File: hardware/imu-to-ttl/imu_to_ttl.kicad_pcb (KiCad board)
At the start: 2 copper layers, 41 x 30 mm, 58 parts, among them J1 BATT IN 2.54 2P, J2 SWD+UART+NRST, J3 J_NECK, J4 J_L, J5 J_R, Q1 AO4407C, U1 STM32G031F8P6, U2 LSM6DSV16XTR, U3 SN74LVC2G241DCUR, U4 HT7533-1

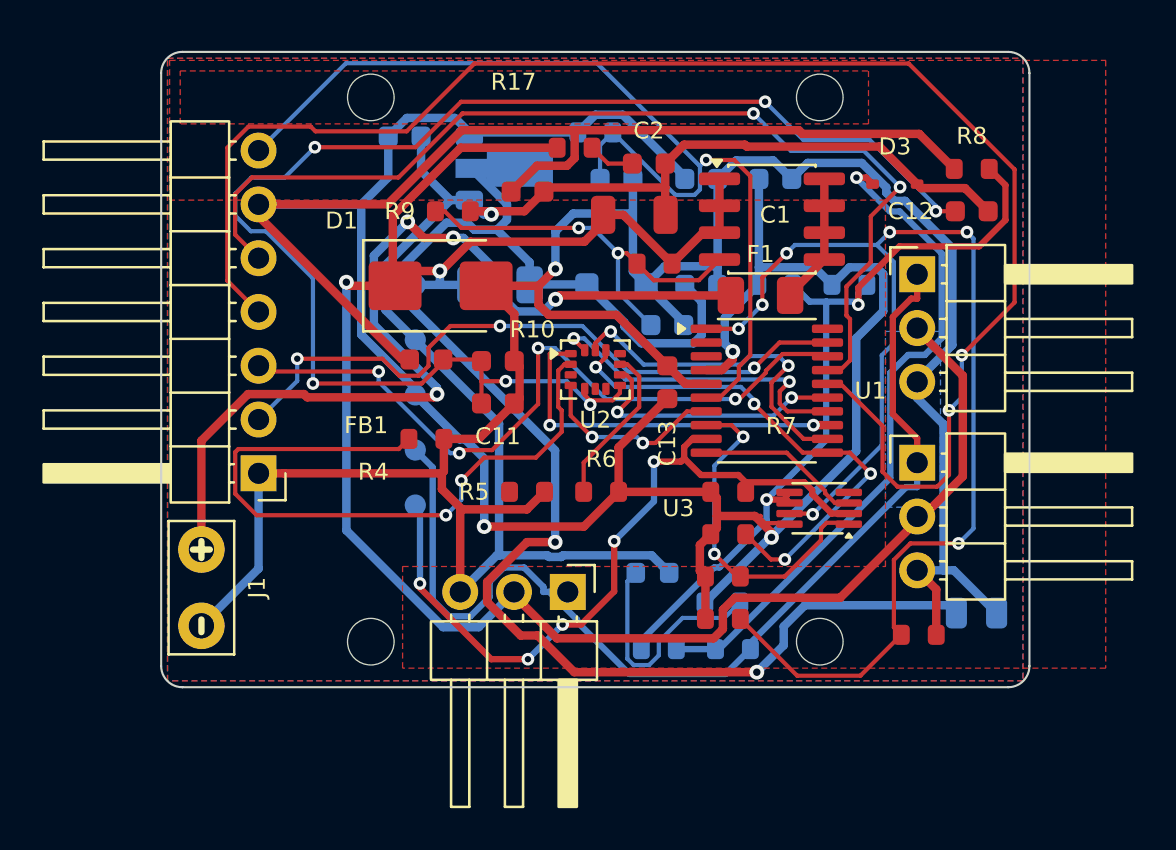
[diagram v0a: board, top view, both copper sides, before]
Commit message: sync: 2026-10-21 日常更新
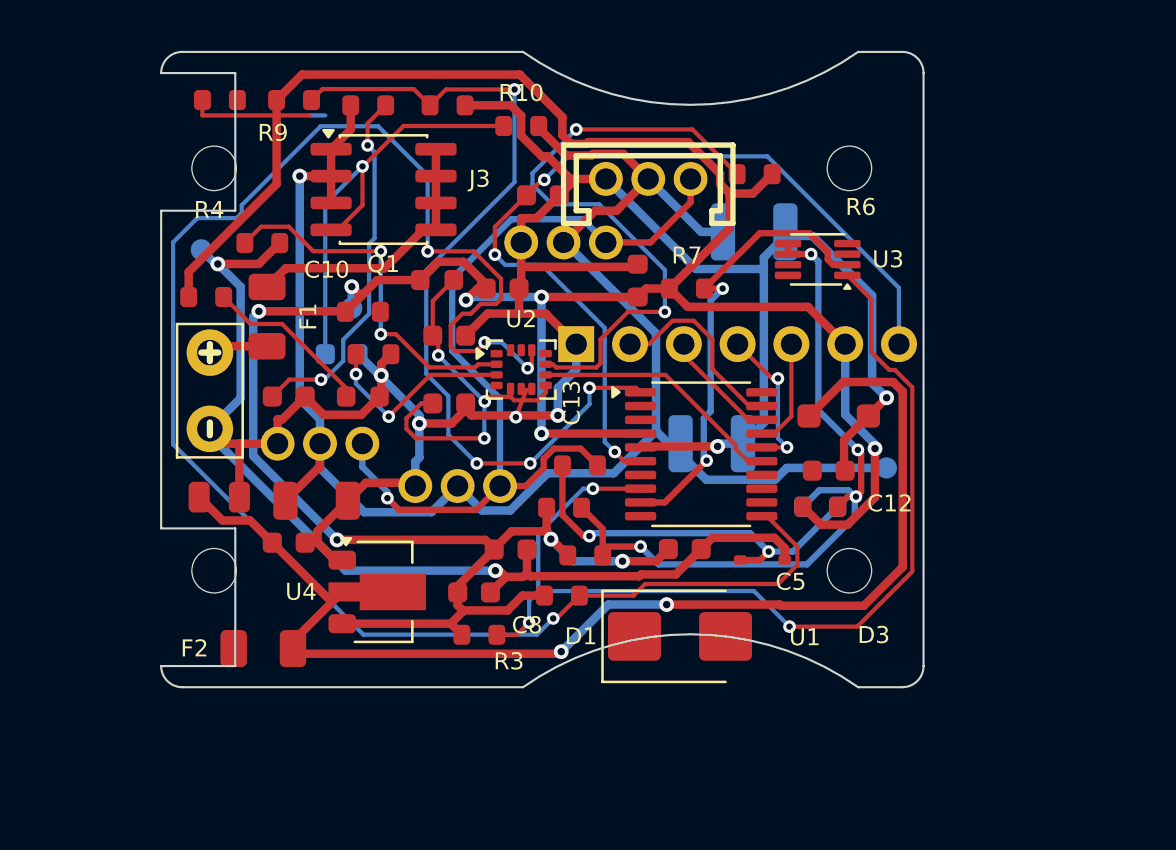
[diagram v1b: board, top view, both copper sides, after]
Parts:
- removed B1, B2, B3, B4: M2, MountingHole_2.2mm_M2
- removed TP4: BUS_DATA, TestPoint_Pad_D1.0mm
- removed TP5: BUS_TX, TestPoint_Pad_D1.0mm
- added C15: 22uF 16V X5R, C_1210_3225Metric, B.Cu at (26.0, 18.5)
- added C16: 22uF 16V X5R, C_1210_3225Metric, B.Cu at (28.0, 8.50)
- added J6: J_HEAD, CONN-TH_B3B-PH-K-S, B.Cu at (7.50, 18.5)
- added M1: M2, MountingHole_2.1mm_M2, F.Cu at (2.50, 5.50)
- added M2: M2, MountingHole_2.1mm_M2, F.Cu at (2.50, 24.5)
- added M3: M2, MountingHole_2.1mm_M2, F.Cu at (32.5, 5.50)
- added M4: M2, MountingHole_2.1mm_M2, F.Cu at (32.5, 24.5)
- C3, C4, C5, C6, C8, C9, D2, F2, LED1, R1, R11, R12, R2, TH1, U4: moved to F.Cu
- J2: footprint PinHeader_1x07_P2.54mm_Horizontal -> PinHeader_1x07_P2.54mm_Vertical; moved to B.Cu
- J3: footprint PinHeader_1x03_P2.54mm_Horizontal -> CONN-TH_B3B-PH-K-S
- J4, J5: footprint PinHeader_1x03_P2.54mm_Horizontal -> CONN-TH_B3B-PH-K-S; moved to B.Cu
- moved C3 36.2 mm to (2.75, 21.0)
- moved R16 33.5 mm to (13.5, 2.52)
- moved R15 31.8 mm to (6.28, 2.27)
- moved R1 28.3 mm to (2.12, 11.6)
- moved C8 24.2 mm to (14.8, 25.5)
- moved J5 23.9 mm to (14.0, 20.5)
- moved TP1 23.9 mm to (34.2, 19.6)
- moved C5 23.5 mm to (24.7, 23.5)
- moved F1 23.3 mm to (5.00, 12.5), turned to 90 degrees
- moved C4 23.0 mm to (6.03, 23.2)
- moved U4 20.9 mm to (10.5, 25.5)
- moved F2 20.5 mm to (4.83, 28.2)
- moved C2 20.2 mm to (6.03, 16.3)
- moved C1 20.2 mm to (7.34, 21.2)
- moved D1 20.0 mm to (24.5, 27.6)
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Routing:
- net UART1_TX: track 74.4 -> 7.20 mm
- net SPI_CS: track 24.2 -> 80.5 mm
- net V3V3_IMU: track 67.9 -> 18.7 mm, vias 6 -> 3
- net UART1_RX: track 48.5 -> 5.15 mm, vias 2 -> 0
- net VBAT_RAW: track 45.2 -> 2.82 mm, vias 4 -> 0
- net TX_EN_N: track 16.3 -> 46.7 mm, vias 2 -> 3
- net SWDIO: track 34.4 -> 5.47 mm, vias 4 -> 0
- net SWCLK: track 31.9 -> 9.18 mm, vias 3 -> 0
- net RX_EN: track 62.4 -> 40.6 mm, vias 7 -> 4
- net OCS_AUX: track 7.69 -> 29.3 mm, vias 0 -> 2
- net GND: track 180.2 -> 158.6 mm, vias 2 -> 8
- net SPI_MISO: track 17.5 -> 0.00 mm, vias 2 -> 0
- net SPI_SCK: track 16.2 -> 0.00 mm, vias 2 -> 0
- net SPI_MOSI: track 15.4 -> 0.00 mm, vias 2 -> 0
- net VBAT_LOGIC: track 71.4 -> 56.2 mm
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- removed copper zone on B.Cu, net GND
- removed copper zone on F.Cu, net GND
- removed copper zone on B.Cu, net VBAT
- removed copper zone on F.Cu, net VBAT
- removed copper zone on F.Cu, net VBAT_RAW
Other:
- board size 41 x 30 mm -> 36 x 30 mm

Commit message: sync: 2026-10-30 日常更新
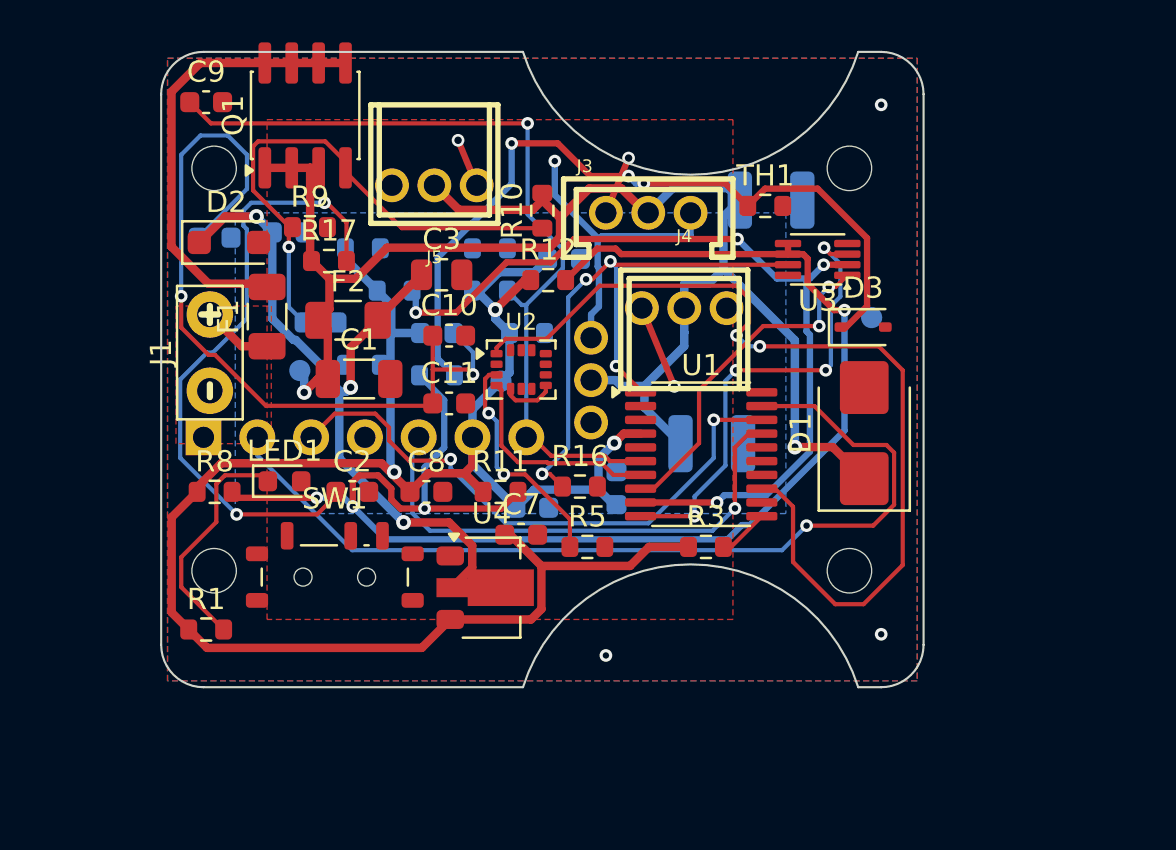
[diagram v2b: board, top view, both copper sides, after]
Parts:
- added SW1: SW SPDT MSK12C02, SW_SPDT_Shouhan_MSK12C02, F.Cu at (8.20, 24.8)
- C12, C13, C4, C5, C6, FB1, R14, R15, R2, R4, R6, R7: moved to B.Cu
- J4, J5: footprint CONN-TH_B3B-PH-K-S -> CONN-TH_S3B-PH-K-S; moved to F.Cu
- moved TP2 31.8 mm to (33.5, 12.5)
- moved C12 31.0 mm to (2.52, 8.78)
- moved D2 29.9 mm to (3.20, 9.00)
- moved R8 28.6 mm to (2.52, 20.8)
- moved TP1 28.1 mm to (6.55, 15.0)
- moved R6 20.6 mm to (9.53, 14.8)
- moved R13 19.1 mm to (13.0, 15.3)
- moved R16 19.1 mm to (19.8, 20.5)
- moved J2 18.1 mm to (2.00, 18.2)
- moved C9 16.5 mm to (2.12, 2.38)
- moved F2 16.0 mm to (8.82, 12.7)
- moved R1 15.7 mm to (2.12, 27.3)
- moved TH1 15.1 mm to (28.5, 7.28)
- moved C3 14.8 mm to (13.2, 10.5)
- moved C5 14.8 mm to (19.0, 9.78)
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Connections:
- R9 pad 2: GND -> PWR_ON_LO
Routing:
- net GND: track 158.6 -> 9.10 mm, vias 8 -> 6
- net SPI_CS: track 80.5 -> 2.41 mm, vias 4 -> 0
- net +3V3: track 148.2 -> 95.8 mm, vias 9 -> 3
- net SPI_MISO: track 0.00 -> 44.6 mm, vias 0 -> 2
- net BUS_LOGIC: track 34.9 -> 71.4 mm
- net SWCLK: track 9.18 -> 43.3 mm, vias 0 -> 1
- net TX_EN_N: track 46.7 -> 16.2 mm, vias 3 -> 2
- net OCS_AUX: track 29.3 -> 0.00 mm, vias 2 -> 0
- net BUS_DATA: track 40.5 -> 14.9 mm
- net VBAT_LOGIC: track 56.2 -> 34.0 mm, vias 2 -> 3
- net SWDIO: track 5.47 -> 27.6 mm, vias 0 -> 2
- net MCU_RX: track 0.00 -> 22.1 mm, vias 0 -> 4
- net V3V3_IMU: track 18.7 -> 40.4 mm, vias 3 -> 2
- net BUS_TX: track 22.0 -> 41.2 mm, vias 2 -> 4
- net UART1_RX: track 5.15 -> 24.1 mm, vias 0 -> 1
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- added copper zone on B.Cu, net GND
- added copper zone on F.Cu, net GND
- added copper zone on B.Cu, net VBAT
- added copper zone on F.Cu, net VBAT
- added copper zone on F.Cu, net VBAT_RAW
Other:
- outline, holes or cut-outs redrawn

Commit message: sync: 2026-10-30 日常更新
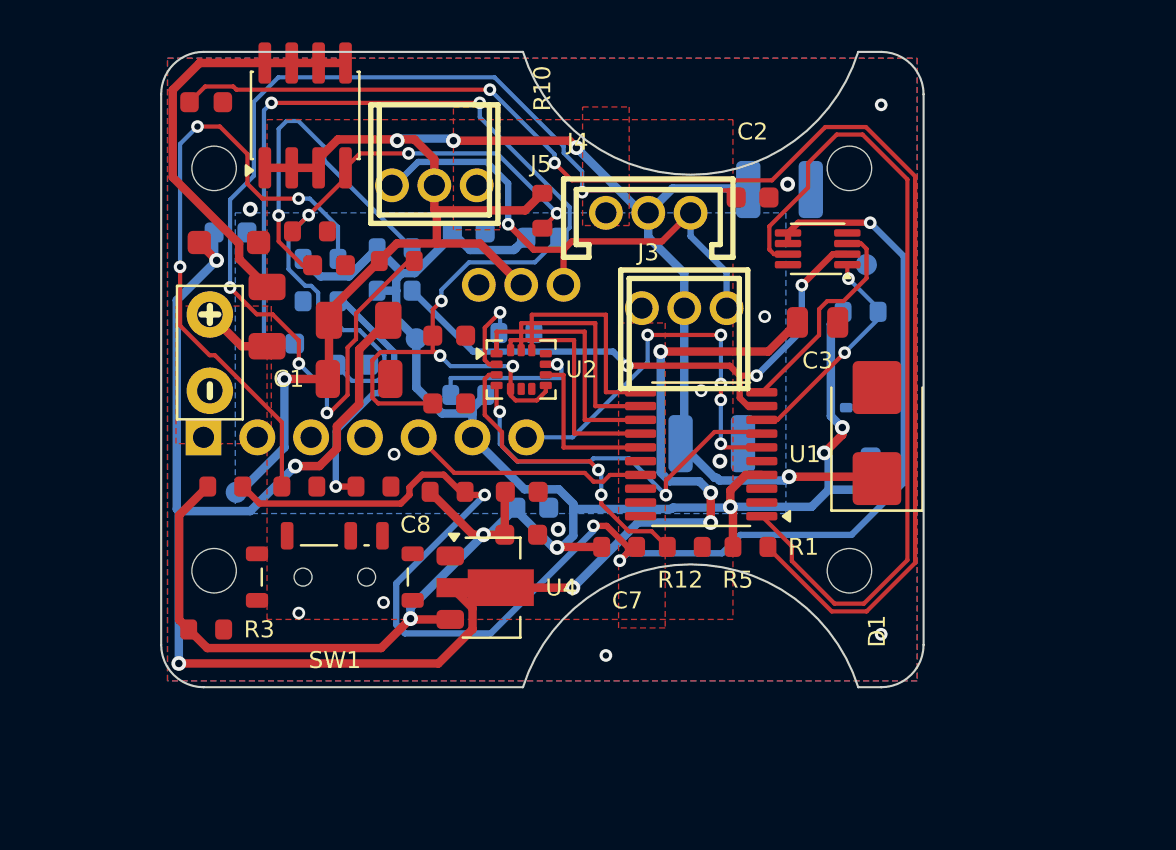
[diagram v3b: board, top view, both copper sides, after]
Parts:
- D3: moved to B.Cu
- moved R1 26.0 mm to (27.8, 23.4)
- moved R3 23.9 mm to (2.12, 27.3)
- moved C2 23.5 mm to (27.9, 6.88)
- moved TH1 22.8 mm to (10.0, 20.5)
- moved LED1 18.3 mm to (2.12, 2.38)
- moved C3 17.9 mm to (31.0, 12.8)
- moved R14 15.8 mm to (33.0, 12.3)
- moved R16 13.2 mm to (6.53, 20.5)
- moved R12 13.0 mm to (21.6, 23.4)
- moved C13 12.0 mm to (33.5, 19.9)
- moved C9 9.64 mm to (7.92, 10.1)
- moved FB1 6.73 mm to (18.0, 8.78)
- moved R13 6.52 mm to (7.53, 11.8)
- moved TP1 6.49 mm to (3.55, 20.8)
- moved C12 5.83 mm to (5.53, 13.8)
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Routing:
- net LED_A: track 11.1 -> 66.1 mm, vias 0 -> 2
- net VBAT_LOGIC: track 34.0 -> 85.5 mm, vias 3 -> 7
- net SWCLK: track 43.3 -> 0.00 mm, vias 1 -> 0
- net RX_EN: track 28.0 -> 70.2 mm, vias 4 -> 3
- net SPI_MISO: track 44.6 -> 12.5 mm, vias 2 -> 0
- net SWDIO: track 27.6 -> 0.00 mm, vias 2 -> 0
- net BUS_CLAMP: track 36.9 -> 12.2 mm, vias 3 -> 1
- net VBAT_C2: track 29.4 -> 53.0 mm, vias 2 -> 4
- net V3V3_IMU: track 40.4 -> 54.9 mm, vias 2 -> 5
- net BUS_TX: track 41.2 -> 28.1 mm, vias 4 -> 3
- net UART1_RX: track 24.1 -> 11.5 mm, vias 1 -> 0
- net MCU_RX: track 22.1 -> 10.3 mm, vias 4 -> 0
- net SPI_MOSI: track 0.00 -> 11.0 mm
- net SPI_SCK: track 0.00 -> 10.8 mm
- net BUS_DATA: track 14.9 -> 25.0 mm
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
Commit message: sync: 2026-10-30 日常更新
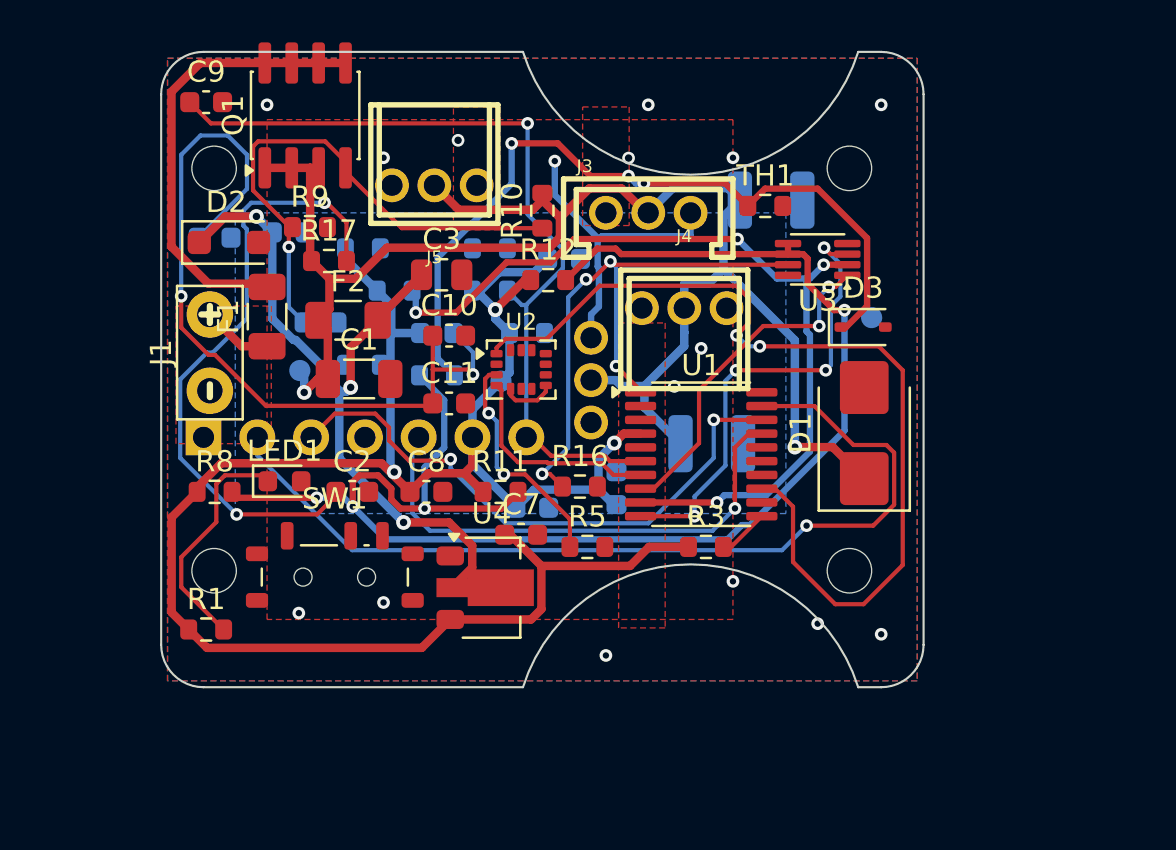
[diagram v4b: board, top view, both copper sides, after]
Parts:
- D3: moved to F.Cu
- moved R1 26.0 mm to (2.12, 27.3)
- moved R3 23.9 mm to (25.7, 23.4)
- moved C2 23.5 mm to (9.03, 20.8)
- moved TH1 22.8 mm to (28.5, 7.28)
- moved LED1 18.3 mm to (5.83, 20.3)
- moved C3 17.9 mm to (13.2, 10.5)
- moved R14 15.8 mm to (17.3, 13.3)
- moved R16 13.2 mm to (19.8, 20.5)
- moved R12 13.0 mm to (18.3, 10.8)
- moved C13 12.0 mm to (21.5, 20.6)
- moved C9 9.64 mm to (2.12, 2.38)
- moved FB1 6.73 mm to (13.0, 13.3)
- moved R13 6.52 mm to (13.0, 15.3)
- moved TP1 6.49 mm to (6.55, 15.0)
- moved C12 5.83 mm to (2.52, 8.78)
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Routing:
- net LED_A: track 66.1 -> 11.1 mm, vias 2 -> 0
- net VBAT_LOGIC: track 85.5 -> 34.0 mm, vias 7 -> 3
- net SWCLK: track 0.00 -> 43.3 mm, vias 0 -> 1
- net RX_EN: track 70.2 -> 28.0 mm, vias 3 -> 4
- net SPI_MISO: track 12.5 -> 44.6 mm, vias 0 -> 2
- net SWDIO: track 0.00 -> 27.6 mm, vias 0 -> 2
- net BUS_CLAMP: track 12.2 -> 36.9 mm, vias 1 -> 3
- net VBAT_C2: track 53.0 -> 29.4 mm, vias 4 -> 2
- net V3V3_IMU: track 54.9 -> 40.4 mm, vias 5 -> 2
- net BUS_TX: track 28.1 -> 41.2 mm, vias 3 -> 4
- net UART1_RX: track 11.5 -> 24.1 mm, vias 0 -> 1
- net MCU_RX: track 10.3 -> 22.1 mm, vias 0 -> 4
- net SPI_MOSI: track 11.0 -> 0.00 mm
- net SPI_SCK: track 10.8 -> 0.00 mm
- net BUS_DATA: track 25.0 -> 14.9 mm
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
